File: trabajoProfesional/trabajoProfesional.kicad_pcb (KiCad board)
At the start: 2 copper layers, 21 parts, among them J1 SYSOUT, J2 BATPositve, J3 BATNegative, J4 GPIO5, J5 GPIO4, J6 GPIO3, J7 GPIO2, J8 GPIO1, U1 TS51224-M000WCSR

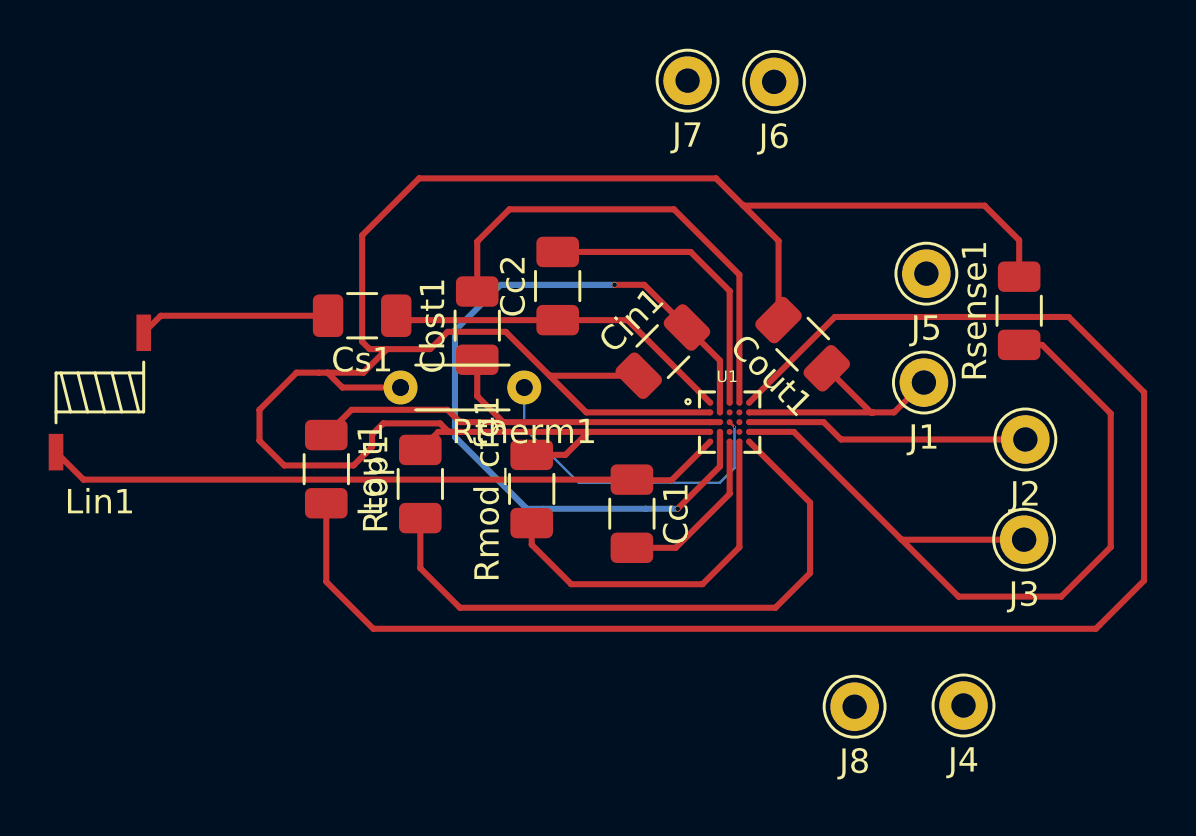
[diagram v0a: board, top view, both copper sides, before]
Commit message: va el parche con el ultimo mod del los pines anulados
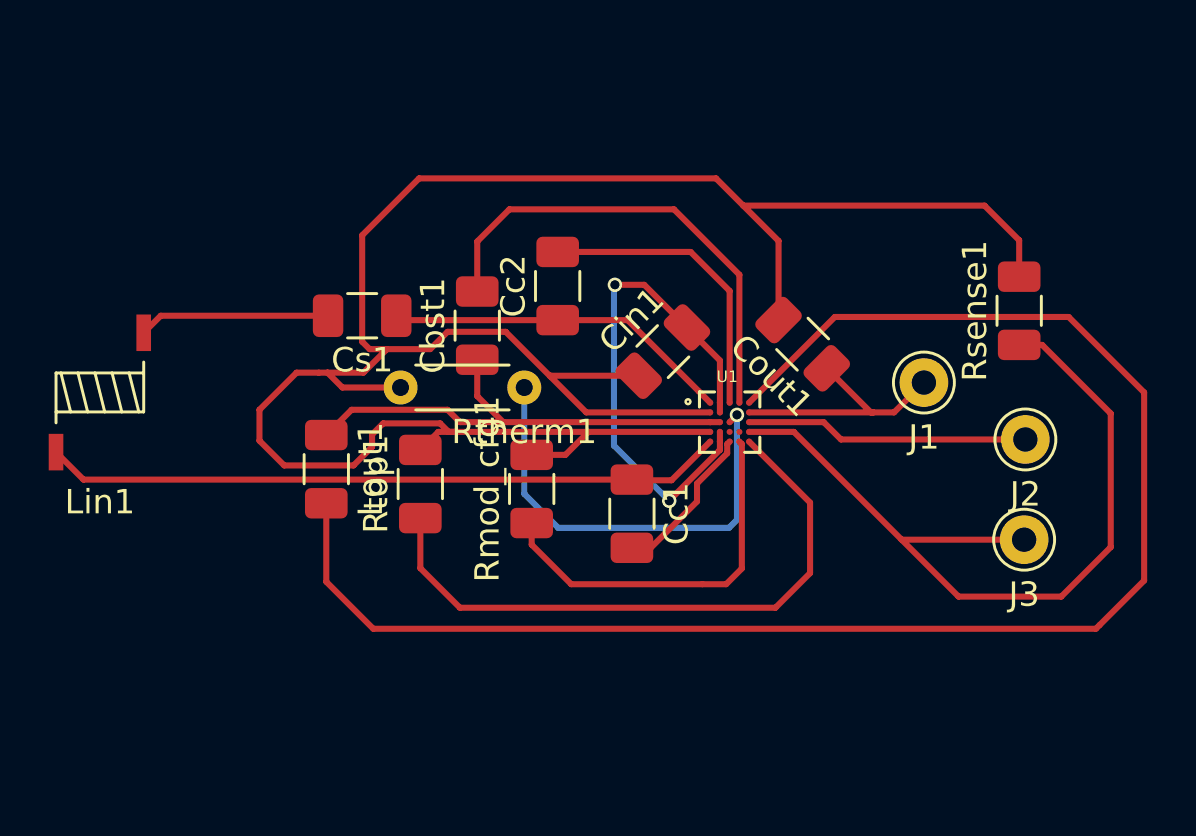
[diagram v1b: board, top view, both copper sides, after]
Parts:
- removed J4: GPIO5, Connector_Pin:Pin_D1.0mm_L10.0mm
- removed J5: GPIO4, Connector_Pin:Pin_D1.0mm_L10.0mm
- removed J6: GPIO3, Connector_Pin:Pin_D1.0mm_L10.0mm
- removed J7: GPIO2, Connector_Pin:Pin_D1.0mm_L10.0mm
- removed J8: GPIO1, Connector_Pin:Pin_D1.0mm_L10.0mm
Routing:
- net Net-(Cin1-Pad2): track 33.7 -> 21.2 mm
- net Net-(Rtherm1-Pad1): track 13.5 -> 18.6 mm
- net Net-(Rmod_cfg1-Pad1): track 15.1 -> 15.7 mm
- net Net-(Cc1-Pad2): track 7.08 -> 6.47 mm
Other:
- net class Default: clearance 0.02 -> 0.0002
- rule trace_clearance: 0.02 -> 0.0002
- rule trace_min: 0.002 -> 0.0002
- rule via_min_drill: 0.0003 -> 0.00003
- rule via_min_size: 0.0004 -> 0.00004
